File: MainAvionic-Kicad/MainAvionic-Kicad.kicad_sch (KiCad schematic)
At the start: 26 parts, among them J1 Conn_01x04_Female, U1 STM32F030C8Tx, U2 Ai-Thinker-Ra-02, U3 L86-M33, U4 BMP180, U5 MPU6050

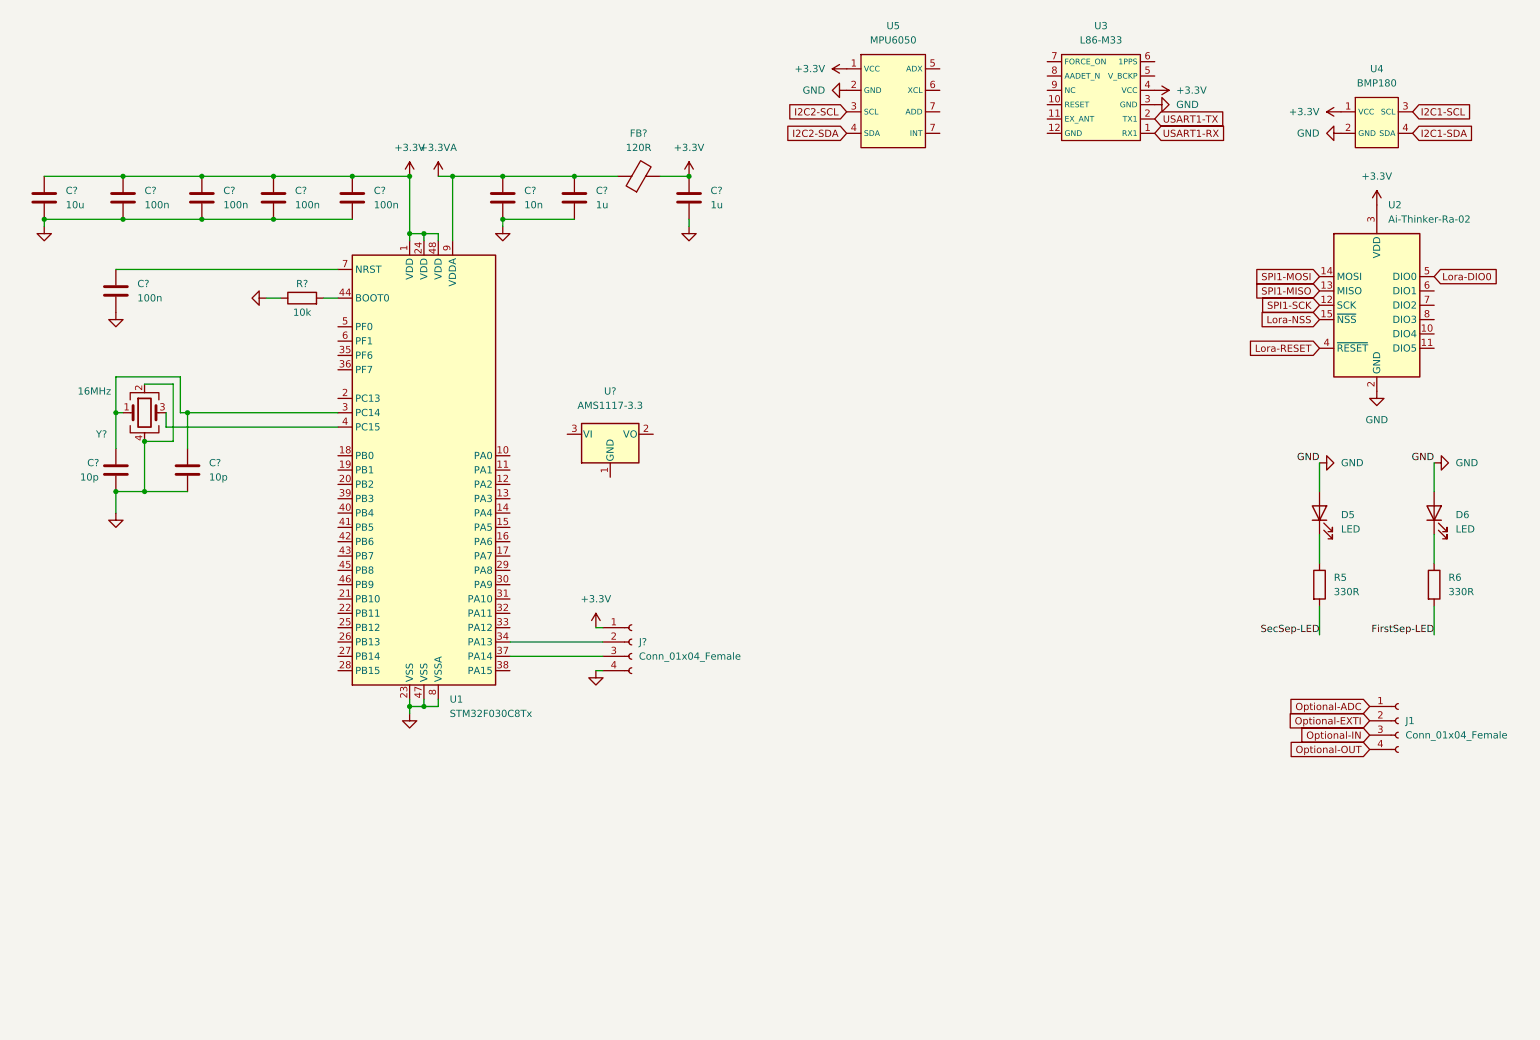
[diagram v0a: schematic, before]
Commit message: update25-11-23
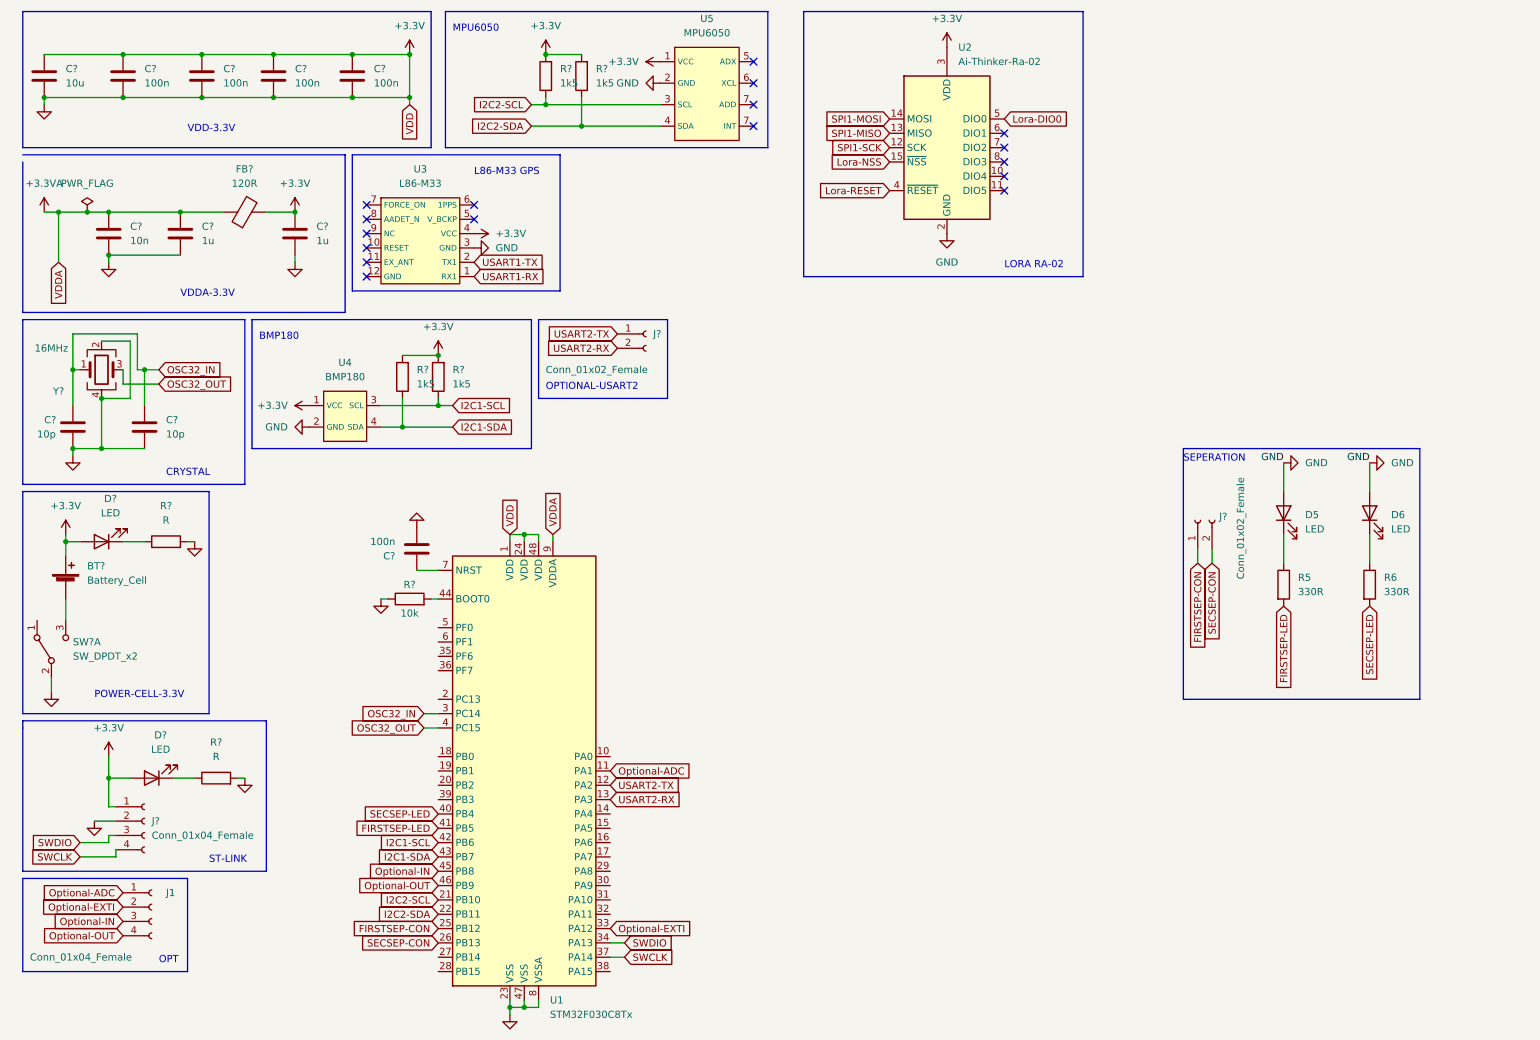
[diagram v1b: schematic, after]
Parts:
- removed C? (x2): 1u, symbol Device:C
- removed C?: 10u, symbol Device:C
- removed C? (x4): 100n, symbol Device:C
- removed C? (x2): 10p, symbol Device:C
- removed C?: 10n, symbol Device:C
- removed FB?: 120R, symbol Device:FerriteBead
- removed J?: Conn_01x04_Female, symbol Connector:Conn_01x04_Female
- removed U?: AMS1117-3.3, Package_TO_SOT_SMD:SOT-223-3_TabPin2, symbol Regulator_Linear:AMS1117-3.3
- removed Y?: 16MHz, symbol Device:Crystal_GND24
- added BT?: Battery_Cell, symbol Device:Battery_Cell
- added C?: 10u, symbol Device:C
- added C? (x2): 10p, symbol Device:C
- added C? (x2): 1u, symbol Device:C
- added C?: 10n, symbol Device:C
- added C? (x4): 100n, symbol Device:C
- added D? (x2): LED, LED_THT:LED_D5.0mm, symbol Device:LED
- added FB?: 120R, symbol Device:FerriteBead
- added J?: Conn_01x04_Female, symbol Connector:Conn_01x04_Female
- added J? (x2): Conn_01x02_Female, symbol Connector:Conn_01x02_Female
- added R? (x2): R, symbol Device:R
- added R? (x4): 1k5, symbol Device:R
- added SW?: SW_DPDT_x2, symbol Switch:SW_DPDT_x2
- added Y?: 16MHz, symbol Device:Crystal_GND24
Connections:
- net FirstSep-LED is gone; now on net SECSEP-LED: R6.2
- net GND is gone; now on net +3.3V: C?.2, D5.2 (A), D6.2 (A), R?.1, U1.23 (VSS), U1.47 (VSS), U1.8 (VSSA), U2.1 (GND), U2.16 (GND), U2.2 (GND), U2.9 (GND), U3.3 (GND), U4.2 (GND), U5.2 (GND)
- net SecSep-LED is gone; now on net FIRSTSEP-LED: R5.2
- net +3.3V: now also BT?.1 (+), C?.1, C?.1, C?.1, C?.1, C?.1, C?.1, C?.2, C?.2, C?.2, C?.2, C?.2, C?.2, C?.2, C?.2, C?.2, C?.2, D?.2 (A), D?.2 (A), FB?.2, J?.1 (Pin_1), J?.2 (Pin_2), R?.2, R?.2, R?.2, R?.2, R?.2, R?.2, SW?.2 (B), Y?.2, Y?.4
- net +3.3VA: now also C?.1, C?.1, FB?.1
- net I2C1-SCL: now also U1.42 (PB6), R?.1
- net I2C1-SDA: now also U1.43 (PB7), R?.1
- net I2C2-SCL: now also U1.21 (PB10), R?.1
- net I2C2-SDA: now also U1.22 (PB11), R?.1
- net Optional-ADC: now also U1.11 (PA1)
- net Optional-EXTI: now also U1.33 (PA12)
- net Optional-IN: now also U1.45 (PB8)
- net Optional-OUT: now also U1.46 (PB9)
- net OSC32_IN: now reaches U1.3 (PC14)
- net OSC32_IN: now also C?.1, C?.1, Y?.1
- net OSC32_OUT: now reaches U1.4 (PC15)
- net OSC32_OUT: now also Y?.3
- net SWDIO: now reaches U1.34 (PA13)
- net SWDIO: now also J?.3 (Pin_3)
- net SWCLK: now reaches U1.37 (PA14)
- net SWCLK: now also J?.4 (Pin_4)
- net USART2-TX: now reaches U1.12 (PA2)
- net USART2-TX: now also J?.1 (Pin_1)
- net USART2-RX: now reaches U1.13 (PA3)
- net USART2-RX: now also J?.2 (Pin_2)
- net FIRSTSEP-CON: now reaches U1.25 (PB12)
- net FIRSTSEP-CON: now also J?.1 (Pin_1)
- net SECSEP-CON: now reaches U1.26 (PB13)
- net SECSEP-CON: now also J?.2 (Pin_2)
- net SECSEP-LED: now reaches U1.40 (PB4)
- net FIRSTSEP-LED: now reaches U1.41 (PB5)
- new net: D?.1 (K), R?.1 (x2)
- new net: BT?.2 (-), SW?.3 (C)
- no-connect marks 0 -> 17
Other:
- note added: "BMP180"
- note added: "CRYSTAL"
- note added: "L86-M33 GPS"
- note added: "LORA RA-02"
- note added: "MPU6050"
- note added: "OPT"
- note added: "OPTIONAL-USART2"
- note added: "POWER-CELL-3.3V"
- note added: "SEPERATION"
- note added: "ST-LINK"
- note added: "VDD-3.3V"
- note added: "VDDA-3.3V"
- moved on the sheet: C?, D5, D6, J1, R5, R6, R?, U1, U2, U3, U4, U5
